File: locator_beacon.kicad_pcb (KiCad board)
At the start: 2 copper layers, 44.9 x 19.9 mm, 23 parts, among them Q1 DMG3406L, Q2 DMP3099, Q3 DMP3099, Q4 DMG3406L, Q5 DMG3406L, U4 MIC2288, U6 XC9140

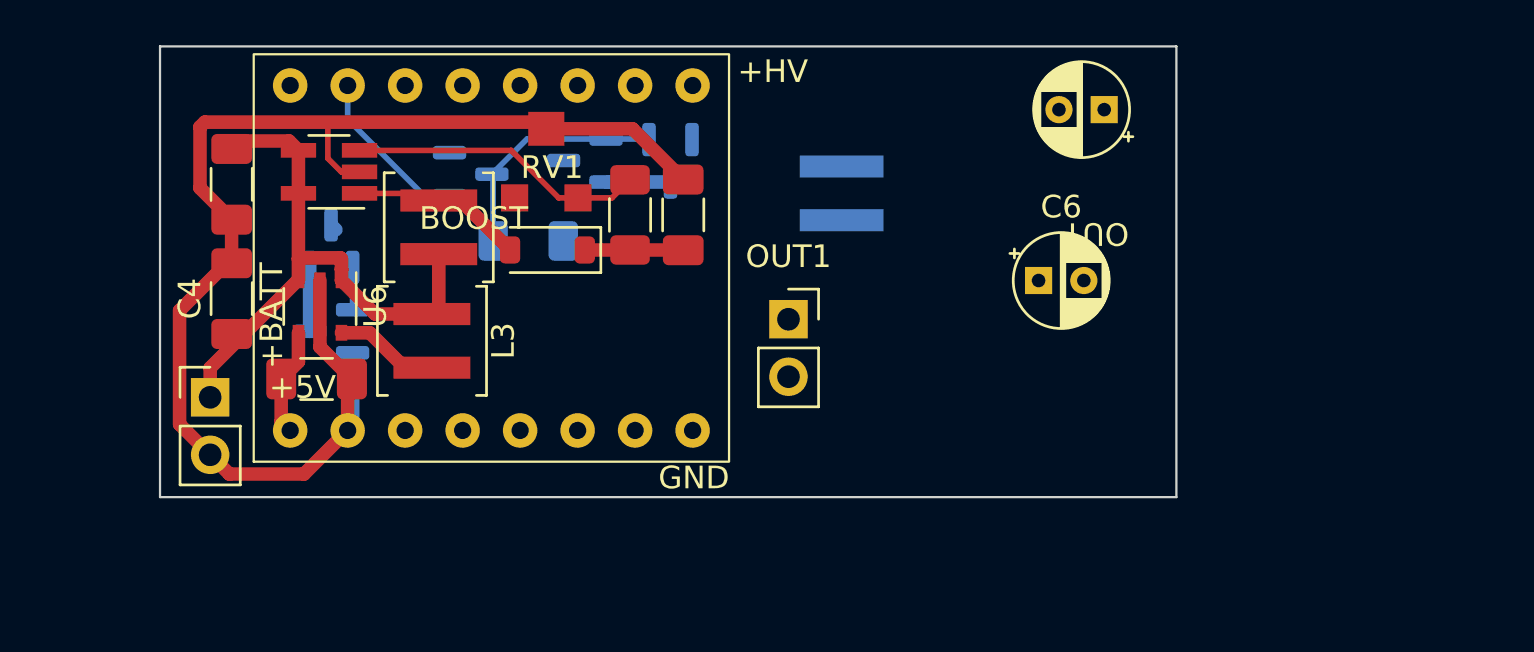
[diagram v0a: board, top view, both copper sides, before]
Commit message: Seems reasonable
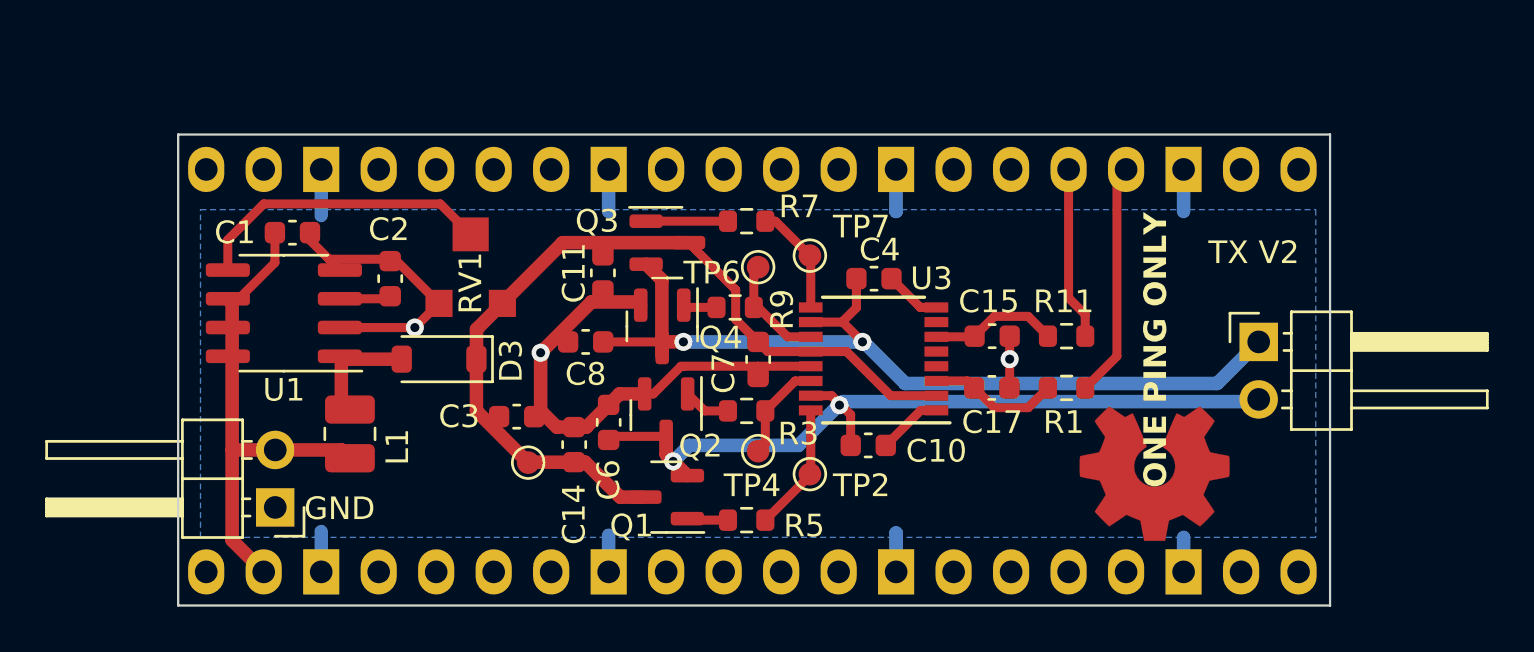
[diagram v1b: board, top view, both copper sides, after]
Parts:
- removed BT1: Battery_Cell, Connector_PinHeader_2.54mm:PinHeader_1x02_P2.54mm_Vertical
- removed C5: 10u, Capacitor_SMD:C_1206_3216Metric_Pad1.33x1.80mm_HandSolder
- removed L2: L, Inductor_SMD:L_Wuerth_MAPI-4030
- removed L3: 4.7u, Inductor_SMD:L_Coilcraft_XAL4030-XXX
- removed OUT1: Speaker, Connector_PinSocket_2.54mm:PinSocket_1x02_P2.54mm_Vertical
- removed Q5: DMG3406L, Package_TO_SOT_SMD:SOT-23
- removed R16: 100k, Resistor_SMD:R_1206_3216Metric_Pad1.30x1.75mm_HandSolder
- removed U4: MIC2288, Package_TO_SOT_SMD:SOT-23-5_HandSoldering
- removed U6: XC9140, Package_SO:TSOP-5_1.65x3.05mm_P0.95mm
- added C10: 10u, Capacitor_SMD:C_0603_1608Metric, F.Cu at (148.4, 81.5)
- added C11: 10u, Capacitor_SMD:C_0603_1608Metric, F.Cu at (136.7, 73.9)
- added C14: 10u, Capacitor_SMD:C_0603_1608Metric, F.Cu at (135.4, 81.5)
- added C15: 10u, Capacitor_SMD:C_0603_1608Metric, F.Cu at (153.8, 76.7)
- added C17: 10u, Capacitor_SMD:C_0603_1608Metric, F.Cu at (153.8, 79.0)
- added C7: 10u, Capacitor_SMD:C_0603_1608Metric, F.Cu at (143.5, 77.7)
- added C8: 10u, Capacitor_SMD:C_0603_1608Metric, F.Cu at (135.9, 77.0)
- added J1: Conn_01x02, Connector_PinHeader_2.54mm:PinHeader_1x02_P2.54mm_Horizontal, F.Cu at (165.6, 77.0)
- added J2: Conn_01x02, Connector_PinHeader_2.54mm:PinHeader_1x02_P2.54mm_Horizontal, F.Cu at (122.2, 84.3)
- added R11: 2k, Resistor_SMD:R_0603_1608Metric, F.Cu at (157.1, 76.7)
- added R3: 2k, Resistor_SMD:R_0603_1608Metric, F.Cu at (143.0, 80.0)
- added R5: 2k, Resistor_SMD:R_0603_1608Metric, F.Cu at (143.0, 84.8)
- added R7: 2k, Resistor_SMD:R_0603_1608Metric, F.Cu at (143.0, 71.6)
- added R9: 2k, Resistor_SMD:R_0603_1608Metric, F.Cu at (142.5, 75.4)
- added REF**: OSHW-Symbol_6.7x6mm_Copper, Symbol:OSHW-Symbol_6.7x6mm_Copper, F.Cu at (161.0, 82.8)
- added REF**: KiCad-Logo2_12mm_SilkScreen, Symbol:KiCad-Logo2_12mm_SilkScreen, B.Cu at (141.7, 76.7)
- added TP1: +V, TestPoint:TestPoint_Pad_D1.0mm, F.Cu at (133.3, 82.3)
- added TP2: LHI, TestPoint:TestPoint_Pad_D1.0mm, F.Cu at (145.8, 82.8)
- added TP4: LLO, TestPoint:TestPoint_Pad_D1.0mm, F.Cu at (143.5, 81.8)
- added TP6: RLO, TestPoint:TestPoint_Pad_D1.0mm, F.Cu at (143.5, 73.7)
- added TP7: RHI, TestPoint:TestPoint_Pad_D1.0mm, F.Cu at (145.8, 73.2)
- added U13: Pico, custom:rp_pico, B.Cu at (142.2, 79.2)
- added U3: MIC4606, Package_SO:TSSOP-16-1EP_4.4x5mm_P0.65mm, F.Cu at (148.6, 77.7)
- C1: value 4.7u -> C; footprint Capacitor_THT:CP_Radial_D4.0mm_P2.00mm -> Capacitor_SMD:C_0603_1608Metric
- C2: value 4.7u -> 1.5n; footprint Capacitor_SMD:C_1206_3216Metric_Pad1.33x1.80mm_HandSolder -> Capacitor_SMD:C_0603_1608Metric
- C3: footprint Capacitor_SMD:C_1206_3216Metric_Pad1.33x1.80mm_HandSolder -> Capacitor_SMD:C_0603_1608Metric
- C4: value 4.7u -> 10u; footprint Capacitor_SMD:C_1206_3216Metric_Pad1.33x1.80mm_HandSolder -> Capacitor_SMD:C_0603_1608Metric
- C6: value 4.7u -> 10u; footprint Capacitor_THT:CP_Radial_D4.0mm_P2.00mm -> Capacitor_SMD:C_0603_1608Metric
- L1: footprint Inductor_SMD:L_Coilcraft_XAL4030-XXX -> Inductor_SMD:L_1008_2520Metric
- Q1, Q4: value DMG3406L -> DMN6140; moved to F.Cu
- Q2, Q3: value DMP3099 -> DMN6140; moved to F.Cu
- R1: value 100k -> 2k; footprint Resistor_SMD:R_1206_3216Metric_Pad1.30x1.75mm_HandSolder -> Resistor_SMD:R_0603_1608Metric; moved to F.Cu
- U1: value ~ -> MC34063AD; footprint RPi:tiny_2040 -> Package_SO:SOIC-8_3.9x4.9mm_P1.27mm
- moved C1 36.3 mm to (122.9, 72.1), turned to 0 degrees
- moved C4 28.4 mm to (148.6, 74.2), turned to 180 degrees
- moved R1 24.7 mm to (157.1, 79.0), turned to 0 degrees
- moved C6 20.0 mm to (136.9, 80.5), turned to 90 degrees
- moved Q2 16.6 mm to (139.4, 80.2), turned to -90 degrees
- moved Q1 16.5 mm to (139.4, 83.8)
- moved C3 11.6 mm to (132.8, 80.3), turned to 0 degrees
- moved L1 9.93 mm to (125.5, 81.0)
- moved U1 8.27 mm to (122.6, 75.7), turned to 180 degrees
- moved C2 8.15 mm to (127.3, 74.2), turned to 90 degrees
- moved Q4 7.32 mm to (139.3, 76.3)
- moved D3 6.80 mm to (129.4, 77.7)
- moved RV1 5.73 mm to (130.8, 73.7)
- moved Q3 5.15 mm to (139.5, 72.6), turned to 0 degrees
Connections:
- C1 pad 1: Vdrive -> +BATT
- C2 pad 1: +BATT -> Net-(U1-TC)
- C4 pad 1: +BATT -> Net-(U3-AHB)
- C4 pad 2: GND -> /amplifier/OUT_B
- C6 pad 1: Vdrive -> /amplifier/OUT_A
- Q1 pad 1: /SIG_P -> Net-(Q1-G)
- Q1 pad 2: GND -> /amplifier/OUT_A
- Q1 pad 3: /OUT_P -> Vdrive
- Q2 pad 1: /SIG_P -> Net-(Q2-G)
- Q2 pad 2: /OUT_P -> GND
- Q2 pad 3: Vdrive -> /amplifier/OUT_A
- Q3 pad 1: /SIG_M -> Net-(Q3-G)
- Q3 pad 2: /OUT_M -> /amplifier/OUT_B
- Q4 pad 1: /SIG_M -> Net-(Q4-G)
- Q4 pad 3: /OUT_M -> /amplifier/OUT_B
- R1 pad 1: Vdrive -> Net-(U3-BPWM)
- R1 pad 2: /SIG_M -> /amplifier/SIG_IN
- RV1 pad 1: unconnected-(RV1-Pad1) -> GND
- RV1 pad 2: GND -> Net-(U1-Vfb)
- RV1 pad 3: Net-(U4-FB) -> Vdrive
- U1 pad 1: +5V -> Net-(D3-A)
- U1 pad 3: unconnected-(U1-3V3-Pad3) -> Net-(U1-TC)
- U1 pad 4: unconnected-(U1-GP29-Pad4) -> GND
- U1 pad 5: unconnected-(U1-GP28-Pad5) -> Net-(U1-Vfb)
- U1 pad 6: unconnected-(U1-GP27-Pad6) -> +BATT
- U1 pad 7: unconnected-(U1-GP26-Pad7) -> +BATT
- U1 pad 8: GND -> +BATT
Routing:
- net /amplifier/OUT_B: track 0.00 -> 40.3 mm, vias 0 -> 2
- net /amplifier/OUT_A: track 0.00 -> 35.6 mm, vias 0 -> 2
- net Vdrive: track 4.66 -> 38.0 mm
- net Net-(U1-Vfb): track 0.00 -> 13.3 mm
- net Net-(U4-FB): track 13.2 -> 0.00 mm
- net /amplifier/SIG_IN: track 0.00 -> 10.8 mm
- net /SIG_M: track 10.6 -> 0.00 mm
- net GND: track 60.7 -> 51.2 mm, vias 0 -> 3
- net /SIG_P: track 9.26 -> 0.00 mm
- net /amplifier/~{SIG_IN}: track 0.00 -> 7.67 mm
- net Net-(U3-APWM): track 0.00 -> 6.26 mm
- net Net-(U3-BPWM): track 0.00 -> 5.78 mm
- net /amplifier/L_HI: track 0.00 -> 5.68 mm
- net /amplifier/R_LO: track 0.00 -> 4.91 mm
- net /amplifier/R_HI: track 0.00 -> 4.90 mm
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- added copper zone on B.Cu, net GND
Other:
- board size 44.9 x 19.9 mm -> 50.9 x 20.8 mm
- board text added: "ONE PING ONLY"
- board text added: "TX V2"
- board text removed: "+5V"
- board text removed: "+BATT"
- board text removed: "+HV"
- board text removed: "BOOST"
- board text removed: "DAC"
- board text removed: "OUT"
- board text removed: "SHAPER"
